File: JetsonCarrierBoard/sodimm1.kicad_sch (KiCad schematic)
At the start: 4 parts

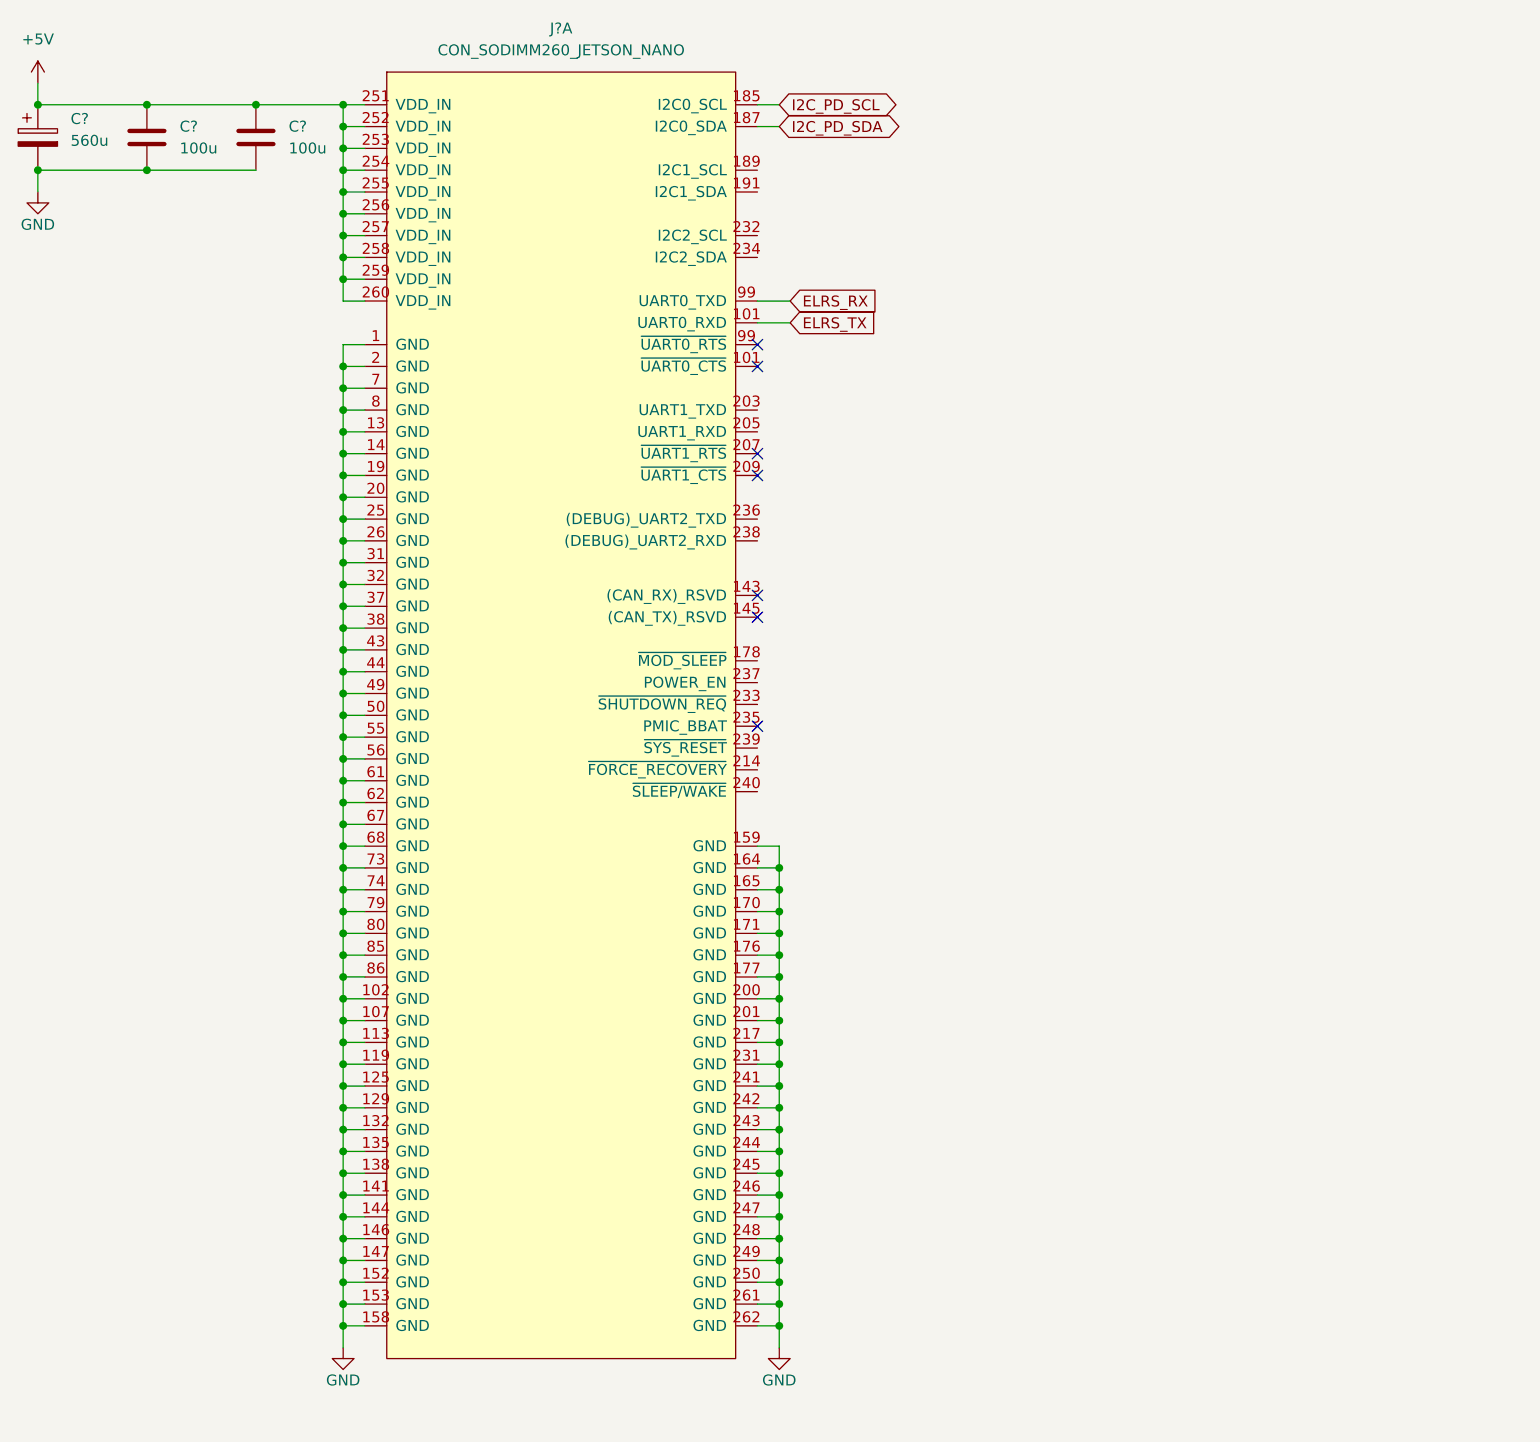
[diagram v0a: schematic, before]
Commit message: Connections
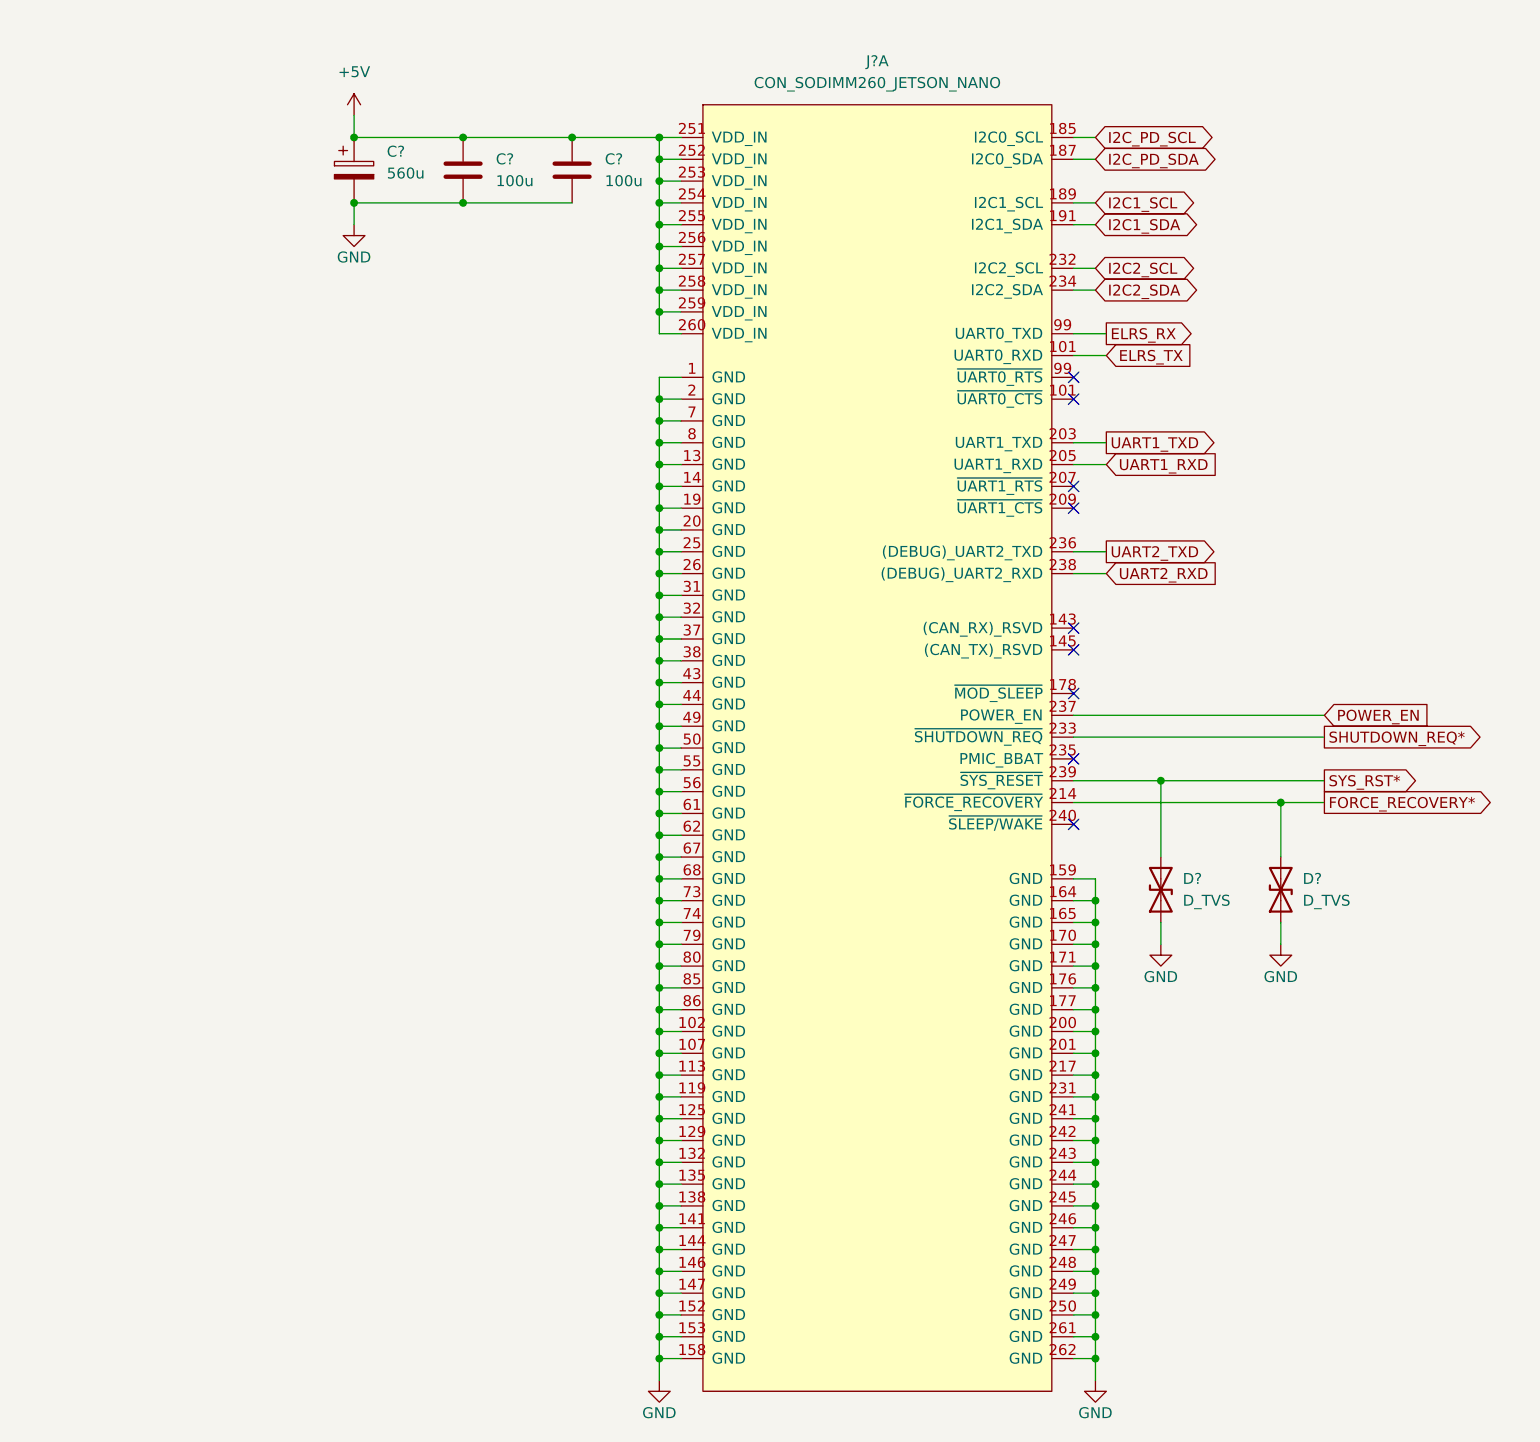
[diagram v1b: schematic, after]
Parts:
- added D? (x2): D_TVS, symbol Device:D_TVS
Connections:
- net GND: now also D?.1 (A1), D?.1 (A1)
- net I2C1_SCL: now reaches J?.189 (I2C1_SCL)
- net I2C1_SDA: now reaches J?.191 (I2C1_SDA)
- net UART1_TXD: now reaches J?.203 (UART1_TXD)
- net UART1_RXD: now reaches J?.205 (UART1_RXD)
- net FORCE_RECOVERY*: now reaches J?.214 (~{FORCE_RECOVERY})
- net FORCE_RECOVERY*: now also D?.2 (A2)
- net I2C2_SCL: now reaches J?.232 (I2C2_SCL)
- net SHUTDOWN_REQ*: now reaches J?.233 (~{SHUTDOWN_REQ})
- net I2C2_SDA: now reaches J?.234 (I2C2_SDA)
- net UART2_TXD: now reaches J?.236 ((DEBUG)_UART2_TXD)
- net POWER_EN: now reaches J?.237 (POWER_EN)
- net UART2_RXD: now reaches J?.238 ((DEBUG)_UART2_RXD)
- net SYS_RST*: now reaches J?.239 (~{SYS_RESET})
- net SYS_RST*: now also D?.2 (A2)
- no-connect marks 7 -> 9
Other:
- moved on the sheet: C?, J?A
